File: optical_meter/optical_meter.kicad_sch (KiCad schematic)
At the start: 13 parts, among them J1 SFP+, J2 SFP+, J3 Conn_01x02_Pin, U1 Pico

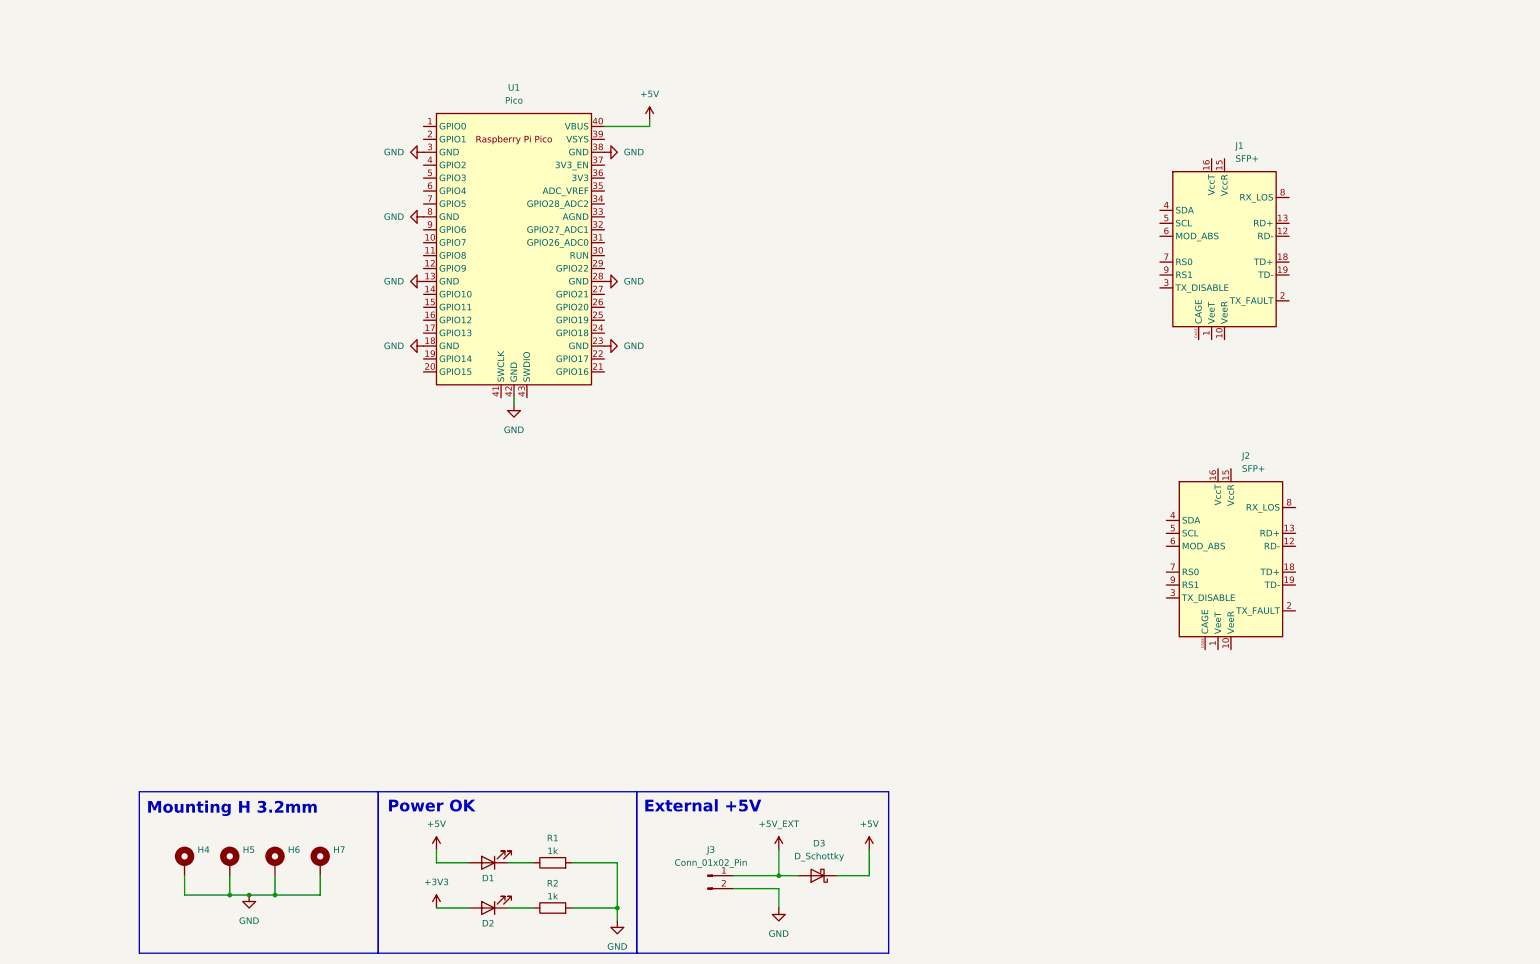
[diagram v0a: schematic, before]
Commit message: Finished schematic (v1.0)
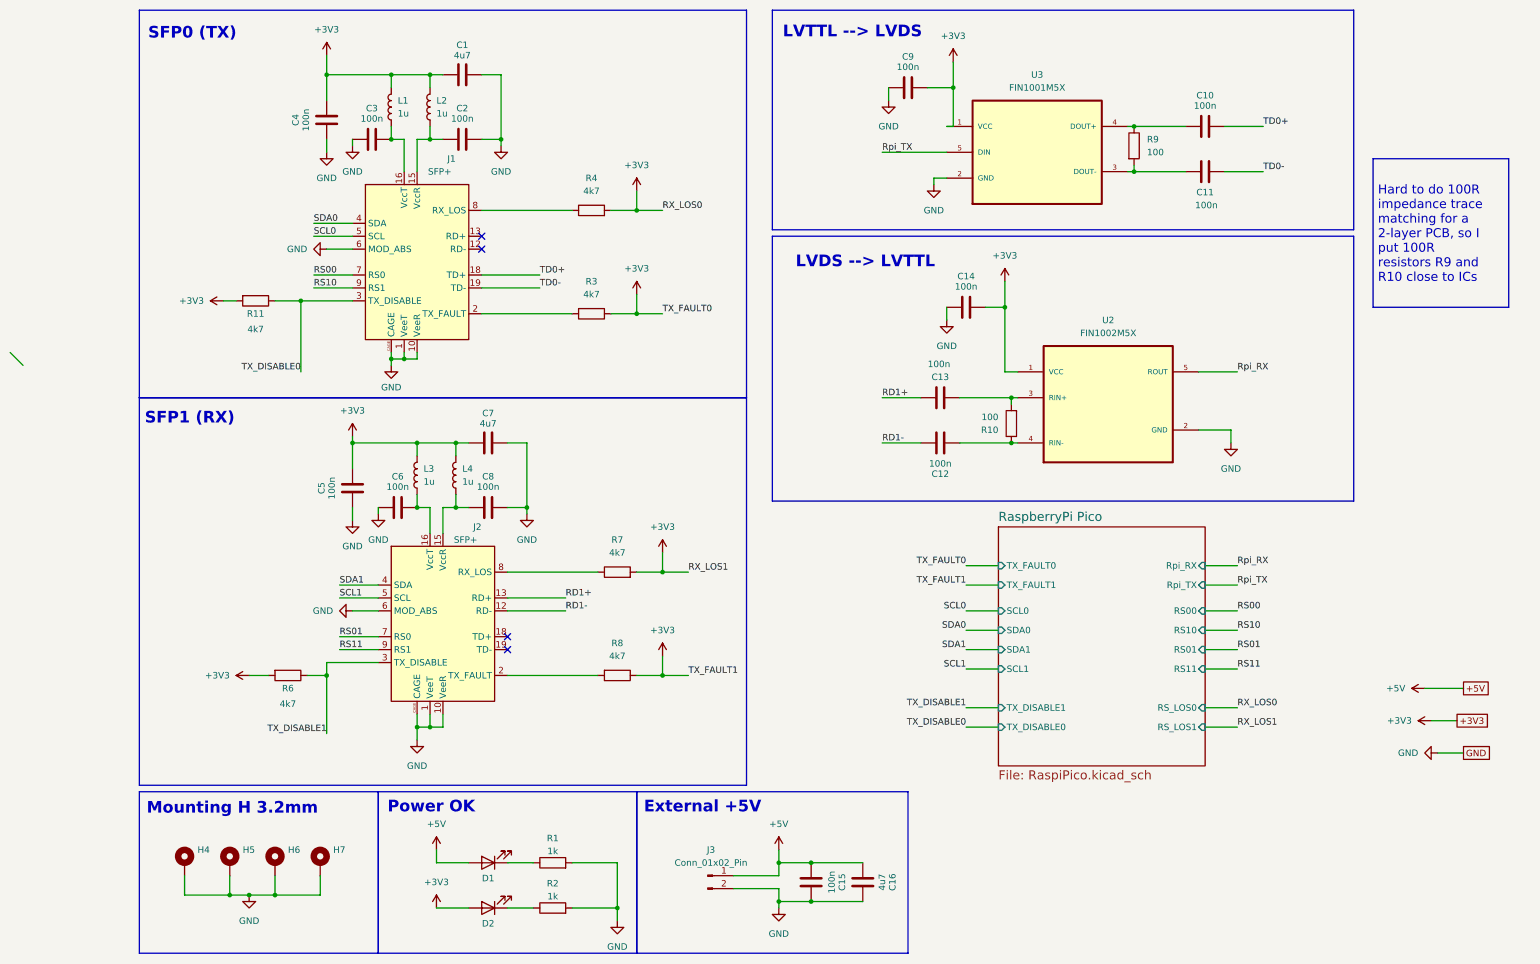
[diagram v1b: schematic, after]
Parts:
- removed D3: D_Schottky, symbol Device:D_Schottky
- removed U1: Pico, MCU_RaspberryPi_and_Boards:RPi_Pico_SMD_TH, symbol MCU_RaspberryPi_and_Boards:Pico
- added C1, C16, C7: 4u7, Capacitor_SMD:C_0603_1608Metric, symbol Device:C
- added C10, C11, C12, C13, C14, C15, C2, C3, C4, C5, C6, C8, C9: 100n, Capacitor_SMD:C_0603_1608Metric, symbol Device:C
- added L1, L2, L3, L4: 1u, Inductor_SMD:L_0805_2012Metric_Pad1.15x1.40mm_HandSolder, symbol Device:L
- added R10, R9: 100, Resistor_SMD:R_0603_1608Metric_Pad0.98x0.95mm_HandSolder, symbol Device:R
- added R11, R3, R4, R6, R7, R8: 4k7, Resistor_SMD:R_0603_1608Metric_Pad0.98x0.95mm_HandSolder, symbol Device:R
- added U2: FIN1002M5X, LVDS_RX_lib:SOT95P280X140-5N, symbol TTL --{gt} LVDS (FIN1002M5X):FIN1002M5X
- added U3: FIN1001M5X, LVDS_RX_lib:SOT95P280X140-5N, symbol LVDS --{gt} TTL (FIN1001M5X):FIN1001M5X
- D1, D2: footprint (none) -> Diode_SMD:D_0603_1608Metric
- J3: footprint (none) -> Connector_PinHeader_2.54mm:PinHeader_1x02_P2.54mm_Vertical
- R1, R2: footprint (none) -> Resistor_SMD:R_0603_1608Metric_Pad0.98x0.95mm_HandSolder
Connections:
- net +5V_EXT is gone; now on net +5V: J3.1 (Pin_1)
- net +3V3: now also C1.1, C14.2, C4.2, C5.2, C7.1, C9.2, L1.2, L2.2, L3.2, L4.2, R11.2, R3.1, R4.2, R6.2, R7.2, R8.1, U2.1 (VCC), U3.1 (VCC)
- net +5V: now also C15.1, C16.1
- net GND: now also J1.1 (VeeT), J1.10 (VeeR), J1.11 (VeeR), J1.14 (VeeR), J1.17 (VeeT), J1.20 (VeeT), J1.6 (MOD_ABS), J1.CAGE, J2.1 (VeeT), J2.10 (VeeR), J2.11 (VeeR), J2.14 (VeeR), J2.17 (VeeT), J2.20 (VeeT), J2.6 (MOD_ABS), J2.CAGE, C1.2, C14.1, C15.2, C16.2, C2.2, C3.1, C4.1, C5.1, C6.1, C7.2, C8.2, C9.1, U2.2 (GND), U3.2 (GND)
- net at J1.15 (VccR): now also C2.1, L2.1
- net at J1.16 (VccT): now also C3.2, L1.1
- net TD0+: now reaches J1.18 (TD+)
- net TD0+: now also C10.2
- net TD0-: now reaches J1.19 (TD-)
- net TD0-: now also C11.2
- net at J1.2 (TX_FAULT): now also R3.2
- net TX_DISABLE0: now reaches J1.3 (TX_DISABLE)
- net TX_DISABLE0: now also R11.1
- net SDA0: now reaches J1.4 (SDA)
- net SCL0: now reaches J1.5 (SCL)
- net RS00: now reaches J1.7 (RS0)
- net at J1.8 (RX_LOS): now also R4.1
- net RS10: now reaches J1.9 (RS1)
- net RD1-: now reaches J2.12 (RD-)
- net RD1-: now also C12.2
- net RD1+: now reaches J2.13 (RD+)
- net RD1+: now also C13.2
- net at J2.15 (VccR): now also C8.1, L4.1
- net at J2.16 (VccT): now also C6.2, L3.1
- net at J2.2 (TX_FAULT): now also R8.2
- net TX_DISABLE1: now reaches J2.3 (TX_DISABLE)
- net TX_DISABLE1: now also R6.1
- net SDA1: now reaches J2.4 (SDA)
- net SCL1: now reaches J2.5 (SCL)
- net RS01: now reaches J2.7 (RS0)
- net at J2.8 (RX_LOS): now also R7.1
- net RS11: now reaches J2.9 (RS1)
- new net: C10.1, R9.1, U3.4 (DOUT+)
- new net: C11.1, R9.2, U3.3 (DOUT-)
- new net: C12.1, R10.1, U2.4 (RIN-)
- new net: C13.1, R10.2, U2.3 (RIN+)
- new net Rpi_RX: U2.5 (ROUT)
- new net Rpi_TX: U3.5 (DIN)
- no-connect marks 0 -> 4
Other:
- added sheet RaspberryPi Pico (RaspiPico.kicad_sch)
- note added: "LVDS --> LVTTL"
- note added: "LVTTL --> LVDS"
- note added: "SFP0 (TX)"
- note added: "SFP1 (RX)"
- moved on the sheet: J1
